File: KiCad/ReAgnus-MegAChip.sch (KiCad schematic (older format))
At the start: 24 parts, among them J1 Conn_01x03, J3 Conn_02x01, J4 Conn_01x01, J5 Conn_01x01, J6 Conn_01x01, J7 Conn_01x01, U1 PLCC-84-Plug, U2 LM1117-3.3, U3 SN74CBTD16210, U4 SN74CBTD16210, U5 SN74CBTD16210, U6 SN74CBTD16210, U8 74LVC1G07, U9 Agnus_TH_plug_pins

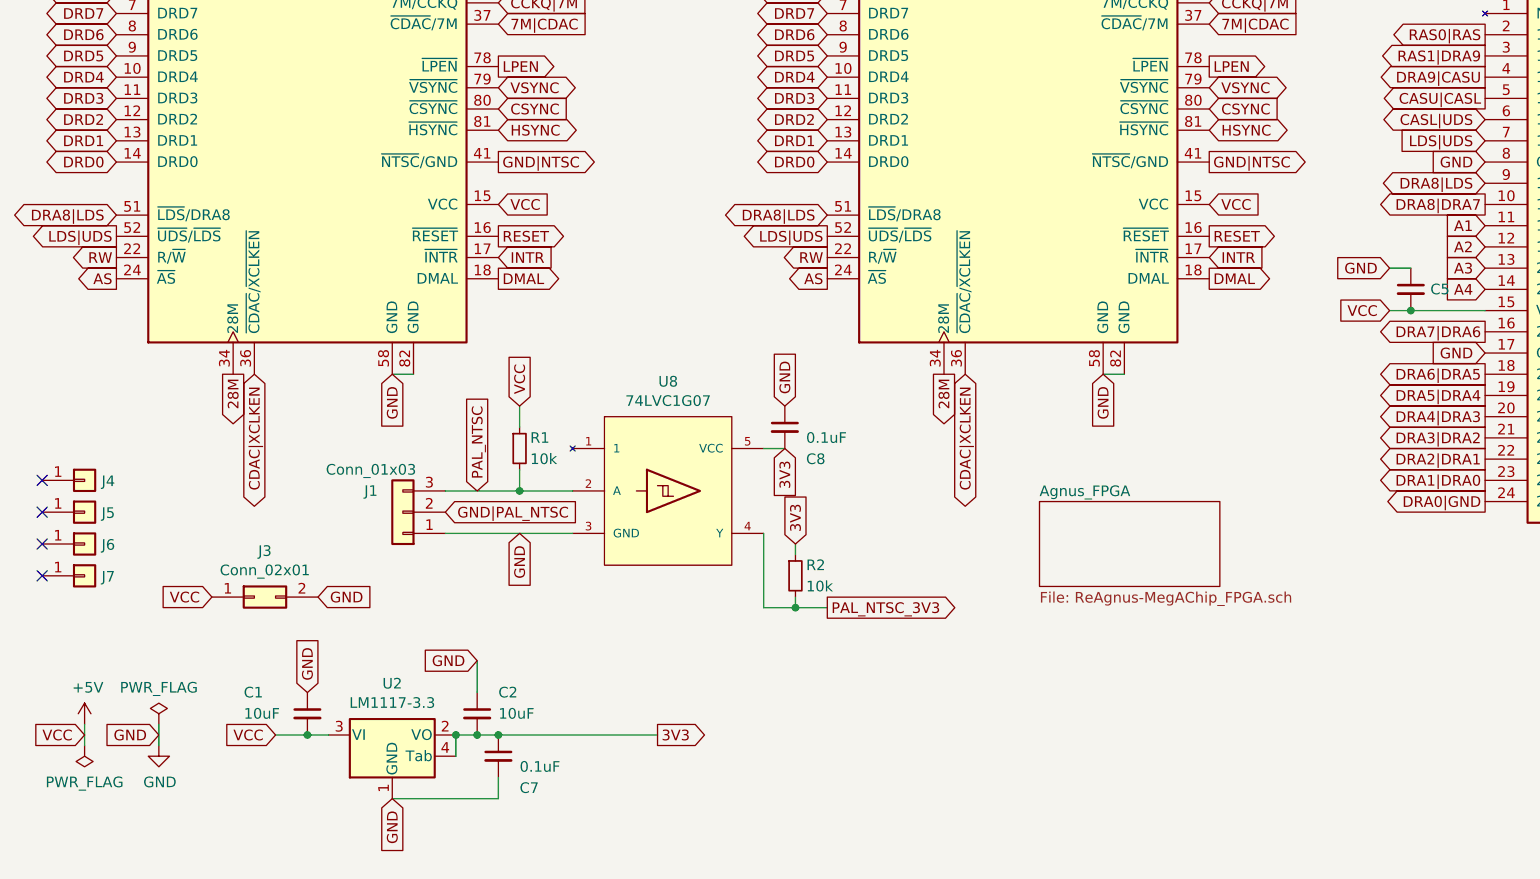
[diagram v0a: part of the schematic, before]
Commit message: more routing and placing components
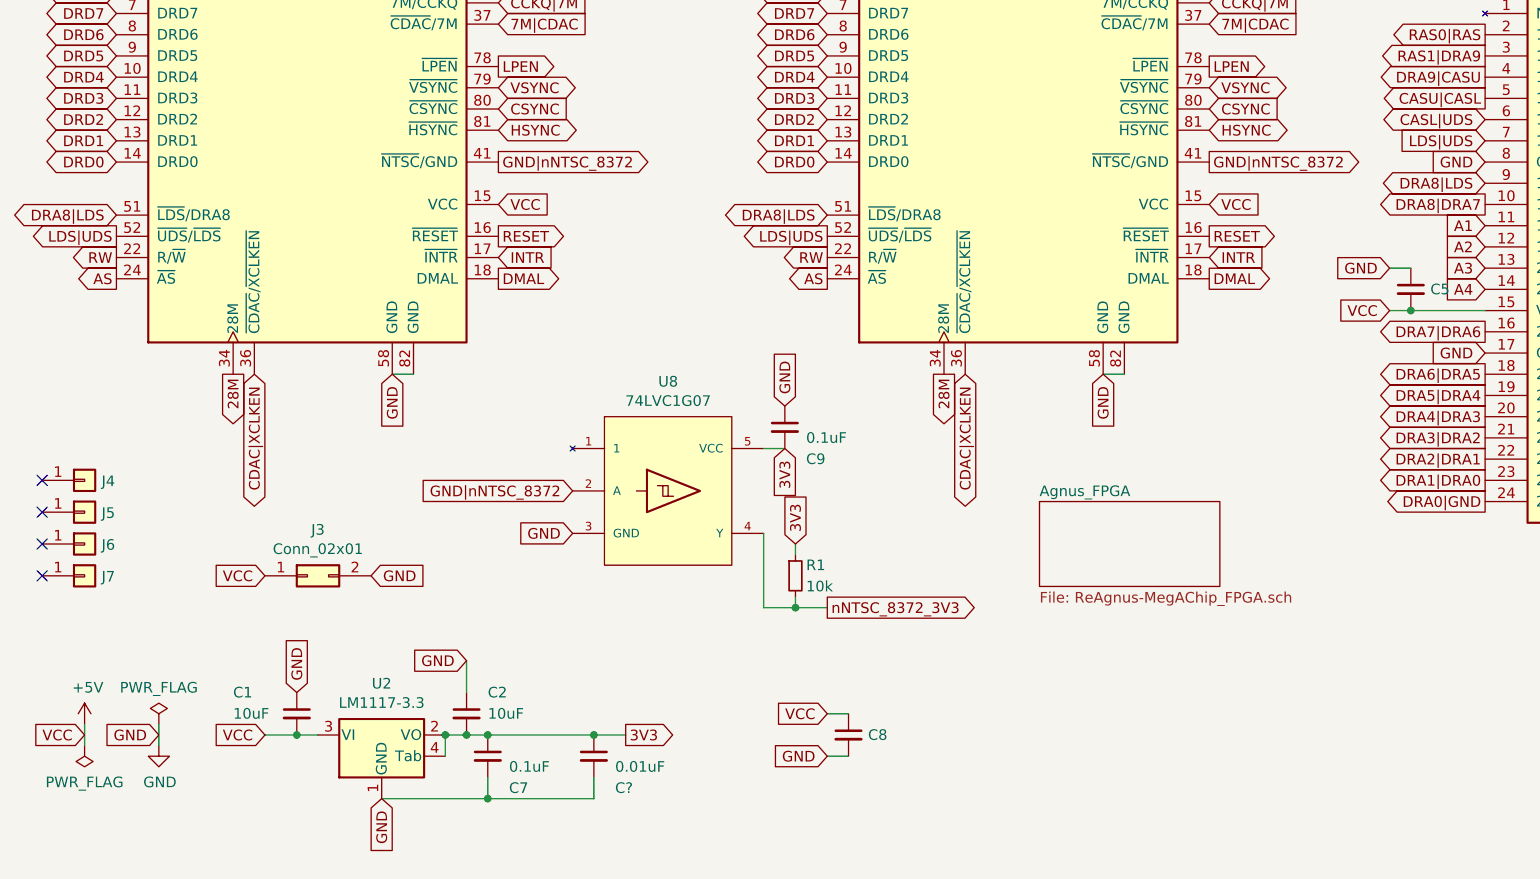
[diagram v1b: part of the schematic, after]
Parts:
- removed J1: Conn_01x03, Connector_PinHeader_2.54mm:PinHeader_1x03_P2.54mm_Vertical, symbol Connector_Generic:Conn_01x03
- removed R1: 10k, Resistor_SMD:R_0603_1608Metric_Pad1.05x0.95mm_HandSolder, symbol Device:R_Small
- added C8: C_Small, Capacitor_SMD:C_1210_3225Metric_Pad1.42x2.65mm_HandSolder, symbol Device:C_Small
- added C?: 0.01uF, Capacitor_SMD:C_0603_1608Metric_Pad1.05x0.95mm_HandSolder, symbol Device:C_Small
- renumbered C8 to C9, R2 to R1
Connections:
- net PAL_NTSC is gone; now on net GND|nNTSC_8372: U8.2 (A)
- net +5V: now also C8.1
- net 3V3: now also C?.1
- net GND: now also C8.2, C?.2
- net GND|NTSC renamed GND|nNTSC_8372
- net PAL_NTSC_3V3 renamed nNTSC_8372_3V3
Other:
- moved on the sheet: C1, C2, C7, J3, U2
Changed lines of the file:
@@
 L Connector_Generic:Conn_02x01 J3
 U 1 1 60E54D12
-P 1650 6750
-F 0 "J3" H 1700 6967 50  0000 C CNN
-F 1 "Conn_02x01" H 1700 6876 50  0000 C CNN
-F 2 "Connector_PinHeader_2.54mm:PinHeader_2x01_P2.54mm_Vertical" H 1650 6750 50  0001 C CNN
-F 3 "~" H 1650 6750 50  0001 C CNN
-	1    1650 6750
-	1    0    0    -1
-$EndComp
-Text GLabel 1950 6750 2    50   Input ~ 0
+P 1900 6650
+F 0 "J3" H 1950 6867 50  0000 C CNN
+F 1 "Conn_02x01" H 1950 6776 50  0000 C CNN
+F 2 "Connector_PinHeader_2.54mm:PinHeader_2x01_P2.54mm_Vertical" H 1900 6650 50  0001 C CNN
+F 3 "~" H 1900 6650 50  0001 C CNN
+	1    1900 6650
+	1    0    0    -1
+$EndComp
+Text GLabel 2200 6650 2    50   Input ~ 0
 GND
 Wire Wire Line
@@
 L ReAgnus-MegAChip:LM1117-3.3 U2
 U 1 1 632C9030
-P 2300 7400
-F 0 "U2" H 2300 7642 50  0000 C CNN
-F 1 "LM1117-3.3" H 2300 7551 50  0000 C CNN
-F 2 "Package_TO_SOT_SMD:SOT-223" H 2300 7400 50  0001 C CNN
-F 3 "" H 2300 7400 50  0001 C CNN
-	1    2300 7400
+P 2250 7400
+F 0 "U2" H 2250 7642 50  0000 C CNN
+F 1 "LM1117-3.3" H 2250 7551 50  0000 C CNN
+F 2 "Package_TO_SOT_SMD:SOT-223" H 2250 7400 50  0001 C CNN
+F 3 "" H 2250 7400 50  0001 C CNN
+	1    2250 7400
 	1    0    0    -1
 $EndComp
@@
 CASU|CASL
 Text GLabel 2800 4700 2    50   Output ~ 0
-GND|NTSC
+GND|nNTSC_8372
 Text GLabel 9750 4500 0    50   Input ~ 0
 A19
@@
 7M|CDAC
 Text GLabel 4350 6800 2    50   Output ~ 0
-PAL_NTSC_3V3
+nNTSC_8372_3V3
 Text GLabel 4350 3200 0    50   BiDi ~ 0
 DRD15
@@
 CASU|CASL
 Text GLabel 6150 4700 2    50   Output ~ 0
-GND|NTSC
+GND|nNTSC_8372
 Text GLabel 4900 5700 3    50   Output ~ 0
 28M
@@
 Text GLabel 8450 6300 2    50   Input ~ 0
 DRA0_3V3|GND
-Text GLabel 2550 6350 2    50   Input ~ 0
-GND|PAL_NTSC
-Text GLabel 1750 7400 0    50   Input ~ 0
+Text GLabel 1700 7400 0    50   Input ~ 0
 VCC
-Text GLabel 1450 6750 0    50   Input ~ 0
+Text GLabel 1700 6650 0    50   Input ~ 0
 VCC
-Text GLabel 1900 7200 1    50   Input ~ 0
+Text GLabel 1850 7200 1    50   Input ~ 0
 GND
 $Comp
 L Device:C_Small C2
 U 1 1 63947670
-P 2700 7300
+P 2650 7300
 AR Path="/63947670" Ref="C2"  Part="1"
 AR Path="/632D3BDF/63947670" Ref="C?"  Part="1"
 AR Path="/632F104D/63947670" Ref="C?"  Part="1"
-F 0 "C2" H 2800 7400 50  0000 L CNN
-F 1 "10uF" H 2800 7300 50  0000 L CNN
-F 2 "Capacitor_SMD:C_1206_3216Metric_Pad1.42x1.75mm_HandSolder" H 2700 7300 50  0001 C CNN
-F 3 "~" H 2700 7300 50  0001 C CNN
-	1    2700 7300
+F 0 "C2" H 2750 7400 50  0000 L CNN
+F 1 "10uF" H 2750 7300 50  0000 L CNN
+F 2 "Capacitor_SMD:C_1206_3216Metric_Pad1.42x1.75mm_HandSolder" H 2650 7300 50  0001 C CNN
+F 3 "~" H 2650 7300 50  0001 C CNN
+	1    2650 7300
 	1    0    0    -1
 $EndComp
@@
 L Device:C_Small C1
 U 1 1 63949338
-P 1900 7300
+P 1850 7300
 AR Path="/63949338" Ref="C1"  Part="1"
 AR Path="/632D3BDF/63949338" Ref="C?"  Part="1"
 AR Path="/632F104D/63949338" Ref="C?"  Part="1"
-F 0 "C1" H 1600 7400 50  0000 L CNN
-F 1 "10uF" H 1600 7300 50  0000 L CNN
-F 2 "Capacitor_SMD:C_1206_3216Metric_Pad1.42x1.75mm_HandSolder" H 1900 7300 50  0001 C CNN
-F 3 "~" H 1900 7300 50  0001 C CNN
-	1    1900 7300
-	1    0    0    -1
-$EndComp
-Wire Wire Line
-	1750 7400 1900 7400
-Connection ~ 1900 7400
-Wire Wire Line
-	1900 7400 2000 7400
-Text GLabel 2700 7050 0    50   Input ~ 0
-GND
-Wire Wire Line
-	2600 7400 2700 7400
-Wire Wire Line
-	2600 7500 2600 7400
-Connection ~ 2600 7400
-Text GLabel 3550 7400 2    50   Output ~ 0
+F 0 "C1" H 1550 7400 50  0000 L CNN
+F 1 "10uF" H 1550 7300 50  0000 L CNN
+F 2 "Capacitor_SMD:C_1206_3216Metric_Pad1.42x1.75mm_HandSolder" H 1850 7300 50  0001 C CNN
+F 3 "~" H 1850 7300 50  0001 C CNN
+	1    1850 7300
+	1    0    0    -1
+$EndComp
+Wire Wire Line
+	1700 7400 1850 7400
+Connection ~ 1850 7400
+Wire Wire Line
+	1850 7400 1950 7400
+Text GLabel 2650 7050 0    50   Input ~ 0
+GND
+Wire Wire Line
+	2550 7400 2650 7400
+Wire Wire Line
+	2550 7500 2550 7400
+Connection ~ 2550 7400
+Text GLabel 3400 7400 2    50   Output ~ 0
 3V3
-Connection ~ 2700 7400
-Wire Wire Line
-	2700 7400 2800 7400
-Text GLabel 2300 7700 3    50   Input ~ 0
+Connection ~ 2650 7400
+Wire Wire Line
+	2650 7400 2750 7400
+Text GLabel 2250 7700 3    50   Input ~ 0
 GND
 $Comp
 L Device:C_Small C7
 U 1 1 63951D9D
-P 2800 7500
+P 2750 7500
 AR Path="/63951D9D" Ref="C7"  Part="1"
 AR Path="/632D3BDF/63951D9D" Ref="C?"  Part="1"
 AR Path="/632F104D/63951D9D" Ref="C?"  Part="1"
-F 0 "C7" H 2900 7350 50  0000 L CNN
-F 1 "0.1uF" H 2900 7450 50  0000 L CNN
-F 2 "Capacitor_SMD:C_0805_2012Metric_Pad1.15x1.40mm_HandSolder" H 2800 7500 50  0001 C CNN
-F 3 "~" H 2800 7500 50  0001 C CNN
-	1    2800 7500
-	1    0    0    -1
-$EndComp
-Connection ~ 2800 7400
-Wire Wire Line
-	2800 7400 3550 7400
-Wire Wire Line
-	2700 7200 2700 7050
-Wire Wire Line
-	2800 7700 2800 7600
-Wire Wire Line
-	2300 7700 2800 7700
+F 0 "C7" H 2850 7350 50  0000 L CNN
+F 1 "0.1uF" H 2850 7450 50  0000 L CNN
+F 2 "Capacitor_SMD:C_0805_2012Metric_Pad1.15x1.40mm_HandSolder" H 2750 7500 50  0001 C CNN
+F 3 "~" H 2750 7500 50  0001 C CNN
+	1    2750 7500
+	1    0    0    -1
+$EndComp
+Wire Wire Line
+	2650 7200 2650 7050
+Wire Wire Line
+	2750 7700 2750 7600
+Wire Wire Line
+	2250 7700 2750 7700
 Wire Wire Line
 	4050 6800 4200 6800
@@
 	1    0    0    -1
 $EndComp
-$Comp
-L Connector_Generic:Conn_01x03 J1
-U 1 1 631AE53C
-P 2350 6350
-F 0 "J1" H 2500 6250 50  0000 C CNN
-F 1 "Conn_01x03" H 2500 6150 50  0000 C CNN
-F 2 "Connector_PinHeader_2.54mm:PinHeader_1x03_P2.54mm_Vertical" H 2350 6350 50  0001 C CNN
-F 3 "~" H 2350 6350 50  0001 C CNN
-	1    2350 6350
-	-1   0    0    1
-$EndComp
-Wire Wire Line
-	3150 6250 2900 6250
-Text GLabel 2900 6450 3    50   Input ~ 0
-GND
-$Comp
-L Device:C_Small C8
+Text GLabel 3150 6450 0    50   Input ~ 0
+GND
+$Comp
+L Device:C_Small C9
 U 1 1 631B6BE4
 P 4150 5950
-AR Path="/631B6BE4" Ref="C8"  Part="1"
+AR Path="/631B6BE4" Ref="C9"  Part="1"
 AR Path="/632D3BDF/631B6BE4" Ref="C?"  Part="1"
 AR Path="/632F104D/631B6BE4" Ref="C?"  Part="1"
-F 0 "C8" H 4250 5800 50  0000 L CNN
+F 0 "C9" H 4250 5800 50  0000 L CNN
 F 1 "0.1uF" H 4250 5900 50  0000 L CNN
 F 2 "Capacitor_SMD:C_0805_2012Metric_Pad1.15x1.40mm_HandSolder" H 4150 5950 50  0001 C CNN
@@
 Text GLabel 7450 4600 0    50   Input ~ 0
 LDS|UDS
-$Comp
-L Device:R_Small R1
-U 1 1 632802A6
-P 2900 6050
-F 0 "R1" H 2950 6100 50  0000 L CNN
-F 1 "10k" H 2950 6000 50  0000 L CNN
-F 2 "Resistor_SMD:R_0603_1608Metric_Pad1.05x0.95mm_HandSolder" H 2900 6050 50  0001 C CNN
-F 3 "~" H 2900 6050 50  0001 C CNN
-	1    2900 6050
-	1    0    0    -1
-$EndComp
-Connection ~ 2900 6250
 Text GLabel 4200 6500 1    50   Input ~ 0
 3V3
-Wire Wire Line
-	2900 6250 2900 6150
-Wire Wire Line
-	2900 5950 2900 5850
-Text GLabel 2700 6250 1    50   Input ~ 0
-PAL_NTSC
-Text GLabel 2900 5850 1    50   Input ~ 0
-VCC
-Wire Wire Line
-	2550 6250 2900 6250
-Wire Wire Line
-	2550 6450 3150 6450
-$Comp
-L Device:R_Small R2
+$Comp
+L Device:R_Small R1
 U 1 1 6328BA47
 P 4200 6650
-F 0 "R2" H 4250 6700 50  0000 L CNN
+F 0 "R1" H 4250 6700 50  0000 L CNN
 F 1 "10k" H 4250 6600 50  0000 L CNN
 F 2 "Resistor_SMD:R_0603_1608Metric_Pad1.05x0.95mm_HandSolder" H 4200 6650 50  0001 C CNN
@@
 Wire Wire Line
 	4200 6800 4350 6800
+Text GLabel 3150 6250 0    50   Input ~ 0
+GND|nNTSC_8372
+Connection ~ 2750 7400
+Text GLabel 4350 7300 0    50   Input ~ 0
+VCC
+Text GLabel 4350 7500 0    50   Input ~ 0
+GND
+$Comp
+L Device:C_Small C8
+U 1 1 631ACF4A
+P 4450 7400
+AR Path="/631ACF4A" Ref="C8"  Part="1"
+AR Path="/632D3BDF/631ACF4A" Ref="C?"  Part="1"
+AR Path="/632F104D/631ACF4A" Ref="C?"  Part="1"
+F 0 "C8" H 4542 7400 50  0000 L CNN
+F 1 "C_Small" H 4542 7355 50  0001 L CNN
+F 2 "Capacitor_SMD:C_1210_3225Metric_Pad1.42x2.65mm_HandSolder" H 4450 7400 50  0001 C CNN
+F 3 "~" H 4450 7400 50  0001 C CNN
+	1    4450 7400
+	1    0    0    -1
+$EndComp
+Wire Wire Line
+	4350 7300 4450 7300
+Wire Wire Line
+	4350 7500 4450 7500
+$Comp
+L Device:C_Small C?
+U 1 1 631E37EB
+P 3250 7500
+AR Path="/631E37EB" Ref="C?"  Part="1"
+AR Path="/632D3BDF/631E37EB" Ref="C?"  Part="1"
+AR Path="/632F104D/631E37EB" Ref="C?"  Part="1"
+F 0 "C?" H 3350 7350 50  0000 L CNN
+F 1 "0.01uF" H 3350 7450 50  0000 L CNN
+F 2 "Capacitor_SMD:C_0603_1608Metric_Pad1.05x0.95mm_HandSolder" H 3250 7500 50  0001 C CNN
+F 3 "~" H 3250 7500 50  0001 C CNN
+	1    3250 7500
+	1    0    0    -1
+$EndComp
+Wire Wire Line
+	2750 7400 3250 7400
+Wire Wire Line
+	3400 7400 3250 7400
+Connection ~ 3250 7400
+Wire Wire Line
+	2750 7700 3250 7700
+Wire Wire Line
+	3250 7700 3250 7600
+Connection ~ 2750 7700
 $EndSCHEMATC
